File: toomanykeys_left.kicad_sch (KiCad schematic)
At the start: 81 parts, among them U1 TLV61070ADBV, U2 SN74LV1T126DBVR

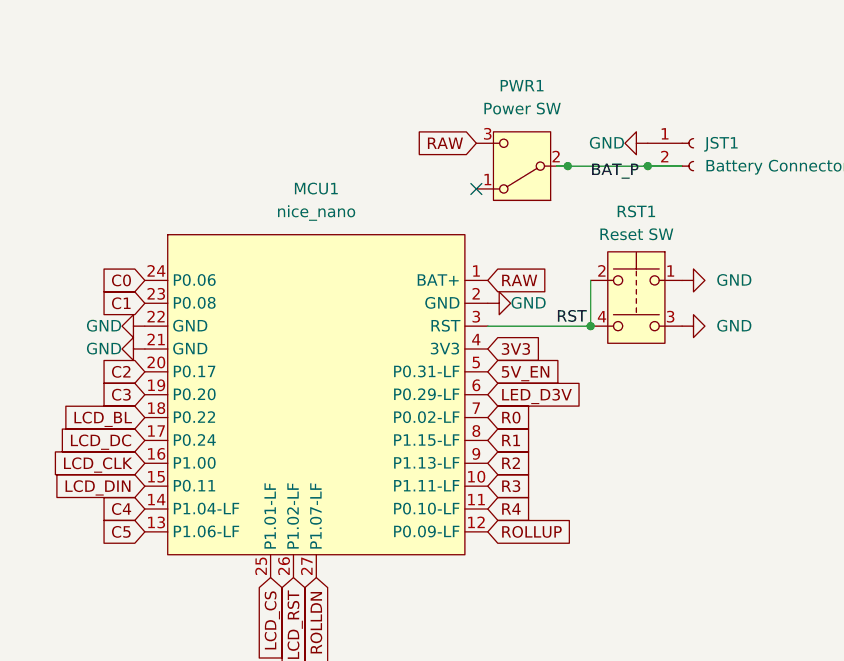
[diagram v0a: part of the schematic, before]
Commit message: Fully route left half. Schematic and PCB both clean!
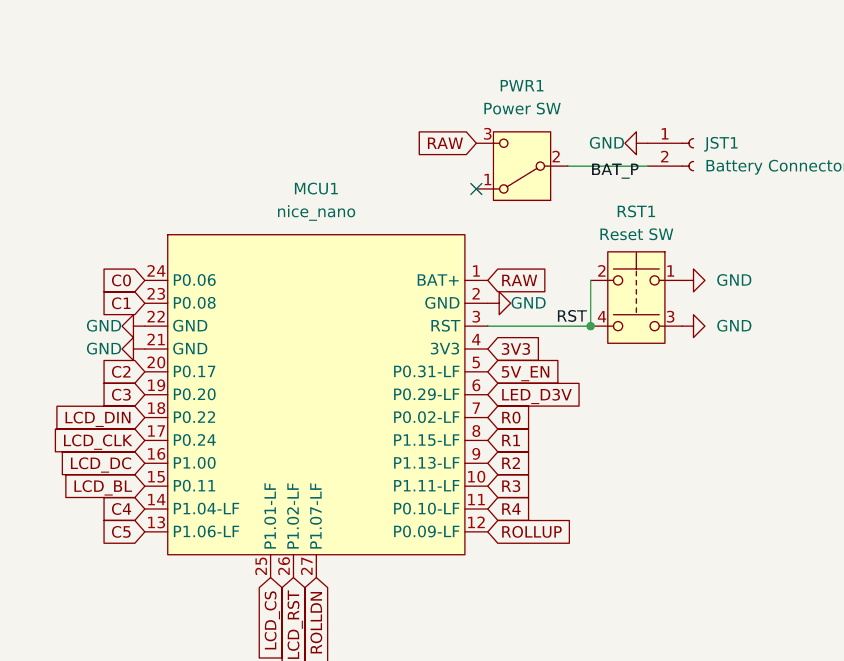
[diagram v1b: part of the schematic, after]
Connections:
- net LCD_BL: now also MCU1.15 (P0.11); no longer MCU1.18 (P0.22)
- net LCD_CLK: now also MCU1.17 (P0.24); no longer MCU1.16 (P1.00)
- net LCD_DC: now also MCU1.16 (P1.00); no longer MCU1.17 (P0.24)
- net LCD_DIN: now also MCU1.18 (P0.22); no longer MCU1.15 (P0.11)
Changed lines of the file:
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@@
 	)
 	(junction
-		(at 85.09 137.16)
-		(diameter 0)
-		(color 0 0 0 0)
-	)
-	(junction
 		(at 52.07 41.91)
 		(diameter 0)
@@
 	)
 	(junction
-		(at 76.2 137.16)
-		(diameter 0)
-		(color 0 0 0 0)
-	)
-	(junction
 		(at 237.49 29.21)
 		(diameter 0)
@@
 	(wire
 		(pts
-			(xy 88.9 137.16) (xy 85.09 137.16)
-		)
-		(stroke
-			(width 0)
-			(type default)
-		)
-	)
-	(wire
-		(pts
 			(xy 29.21 60.96) (xy 46.99 60.96)
 		)
@@
 	(wire
 		(pts
+			(xy 76.2 137.16) (xy 85.09 137.16)
+		)
+		(stroke
+			(width 0)
+			(type default)
+		)
+	)
+	(wire
+		(pts
 			(xy 209.55 147.32) (xy 215.9 147.32)
 		)
@@
 	(wire
 		(pts
-			(xy 76.2 137.16) (xy 85.09 137.16)
-		)
-		(stroke
-			(width 0)
-			(type default)
-		)
-	)
-	(wire
-		(pts
 			(xy 171.45 44.45) (xy 171.45 59.69)
 		)
@@
 	(wire
 		(pts
-			(xy 74.93 137.16) (xy 76.2 137.16)
-		)
-		(stroke
-			(width 0)
-			(type default)
-		)
-	)
-	(wire
-		(pts
 			(xy 95.25 20.32) (xy 95.25 26.67)
 		)
@@
 		)
 	)
-	(global_label "LCD_DC"
-		(shape input)
-		(at 29.21 167.64 180)
-		(fields_autoplaced yes)
-		(effects
-			(font
-				(size 1.27 1.27)
-			)
-			(justify right)
-		)
-		(property "Intersheetrefs" "${INTERSHEET_REFS}"
-			(at 19.1491 167.64 0)
-			(effects
-				(font
-					(size 1.27 1.27)
-				)
-				(justify right)
-				(hide yes)
-			)
-		)
-	)
 	(global_label "5V"
 		(shape input)
@@
 		)
 	)
-	(global_label "LCD_BL"
-		(shape input)
-		(at 29.21 165.1 180)
-		(fields_autoplaced yes)
-		(effects
-			(font
-				(size 1.27 1.27)
-			)
-			(justify right)
-		)
-		(property "Intersheetrefs" "${INTERSHEET_REFS}"
-			(at 19.391 165.1 0)
-			(effects
-				(font
-					(size 1.27 1.27)
-				)
-				(justify right)
-				(hide yes)
-			)
-		)
-	)
 	(global_label "C2"
 		(shape input)
@@
 		)
 	)
-	(global_label "LCD_DIN"
-		(shape input)
-		(at 29.21 172.72 180)
-		(fields_autoplaced yes)
-		(effects
-			(font
-				(size 1.27 1.27)
-			)
-			(justify right)
-		)
-		(property "Intersheetrefs" "${INTERSHEET_REFS}"
-			(at 18.4838 172.72 0)
-			(effects
-				(font
-					(size 1.27 1.27)
-				)
-				(justify right)
-				(hide yes)
-			)
-		)
-	)
 	(global_label "ROLLUP"
 		(shape input)
@@
 		)
 	)
-	(global_label "LCD_CLK"
-		(shape input)
-		(at 29.21 170.18 180)
-		(fields_autoplaced yes)
-		(effects
-			(font
-				(size 1.27 1.27)
-			)
-			(justify right)
-		)
-		(property "Intersheetrefs" "${INTERSHEET_REFS}"
-			(at 18.121 170.18 0)
-			(effects
-				(font
-					(size 1.27 1.27)
-				)
-				(justify right)
-				(hide yes)
-			)
-		)
-	)
 	(global_label "LCD_CS"
 		(shape input)
@@
 		)
 	)
+	(global_label "LCD_DIN"
+		(shape input)
+		(at 29.21 165.1 180)
+		(fields_autoplaced yes)
+		(effects
+			(font
+				(size 1.27 1.27)
+			)
+			(justify right)
+		)
+		(property "Intersheetrefs" "${INTERSHEET_REFS}"
+			(at 18.4838 165.1 0)
+			(effects
+				(font
+					(size 1.27 1.27)
+				)
+				(justify right)
+				(hide yes)
+			)
+		)
+	)
 	(global_label "LED_D3V"
 		(shape input)
@@
 		)
 	)
+	(global_label "LCD_CLK"
+		(shape input)
+		(at 29.21 167.64 180)
+		(fields_autoplaced yes)
+		(effects
+			(font
+				(size 1.27 1.27)
+			)
+			(justify right)
+		)
+		(property "Intersheetrefs" "${INTERSHEET_REFS}"
+			(at 18.121 167.64 0)
+			(effects
+				(font
+					(size 1.27 1.27)
+				)
+				(justify right)
+				(hide yes)
+			)
+		)
+	)
 	(global_label "C1"
 		(shape input)
@@
 				(hide yes)
 			)
+		)
+	)
+	(global_label "LCD_DC"
+		(shape input)
+		(at 29.21 170.18 180)
+		(fields_autoplaced yes)
+		(effects
+			(font
+				(size 1.27 1.27)
+			)
+			(justify right)
+		)
+		(property "Intersheetrefs" "${INTERSHEET_REFS}"
+			(at 19.1491 170.18 0)
+			(effects
+				(font
+					(size 1.27 1.27)
+				)
+				(justify right)
+				(hide yes)
+			)
+		)
+	)
+	(global_label "LCD_BL"
+		(shape input)
+		(at 29.21 172.72 180)
+		(fields_autoplaced yes)
+		(effects
+			(font
+				(size 1.27 1.27)
+			)
+			(justify right)
+		)
+		(property "Intersheetrefs" "${INTERSHEET_REFS}"
+			(at 19.391 172.72 0)
+			(effects
+				(font
+					(size 1.27 1.27)
+				)
+				(justify right)
+				(hide yes)
+			)
